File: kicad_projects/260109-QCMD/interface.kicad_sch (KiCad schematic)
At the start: 43 parts, among them J1 Conn_01x24_Socket, J2 Conn_01x24_Socket, Q1 BSS138, Q2 BSS138, Q3 BSS138, U3 LM2735YMF, U4 MIC5219-5.0YM5, U5 MIC5219-5.0YM5, U6 MIC5219-5.0YM5

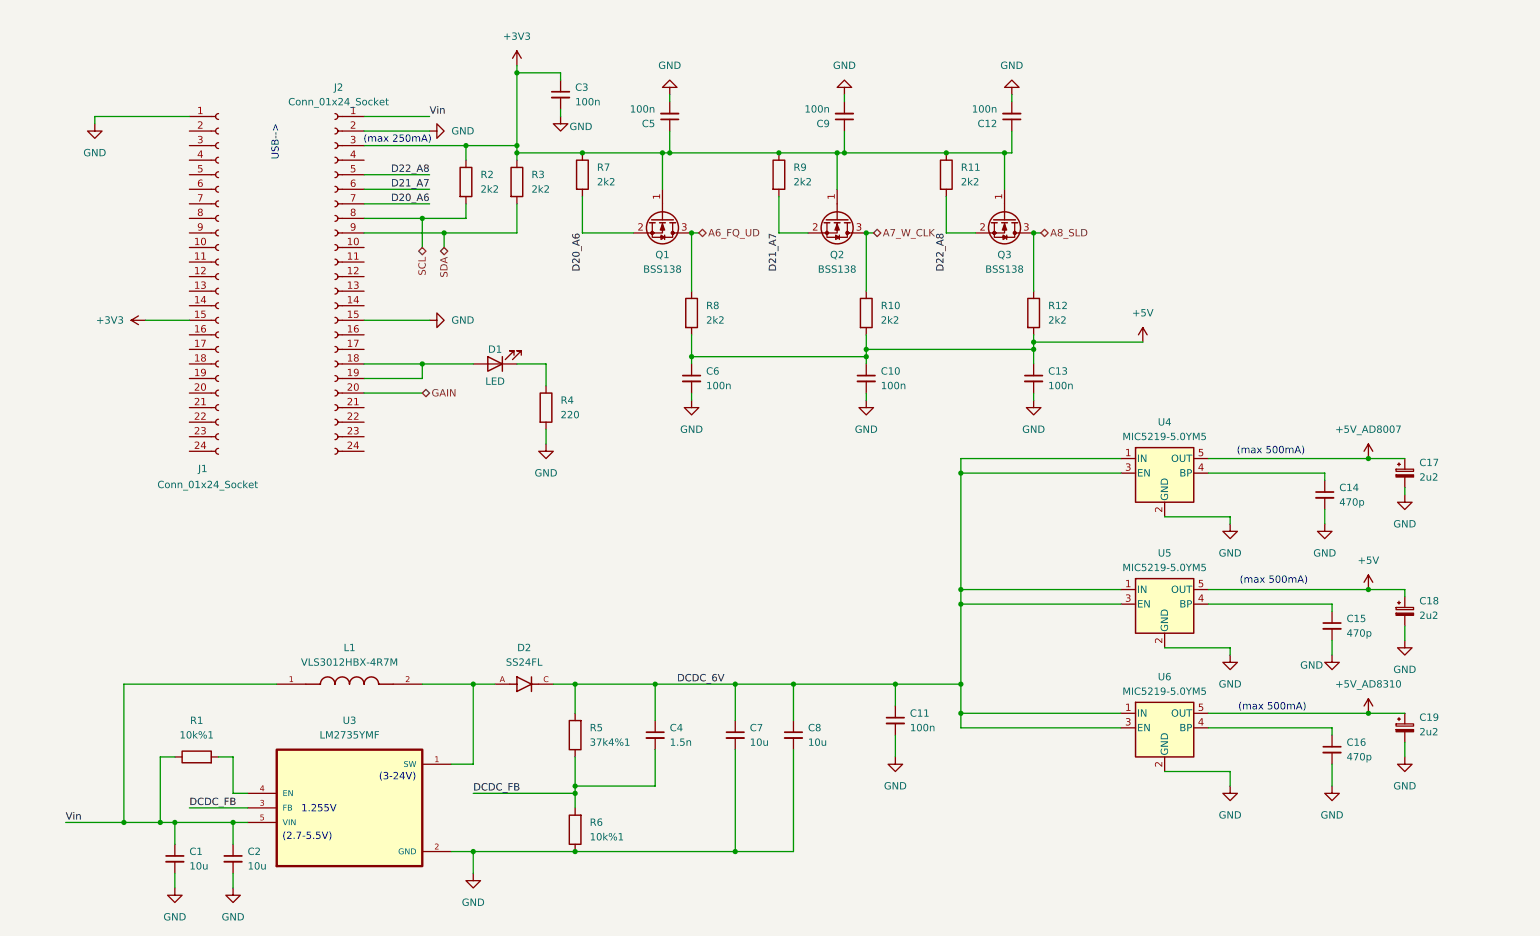
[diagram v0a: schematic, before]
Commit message: regular
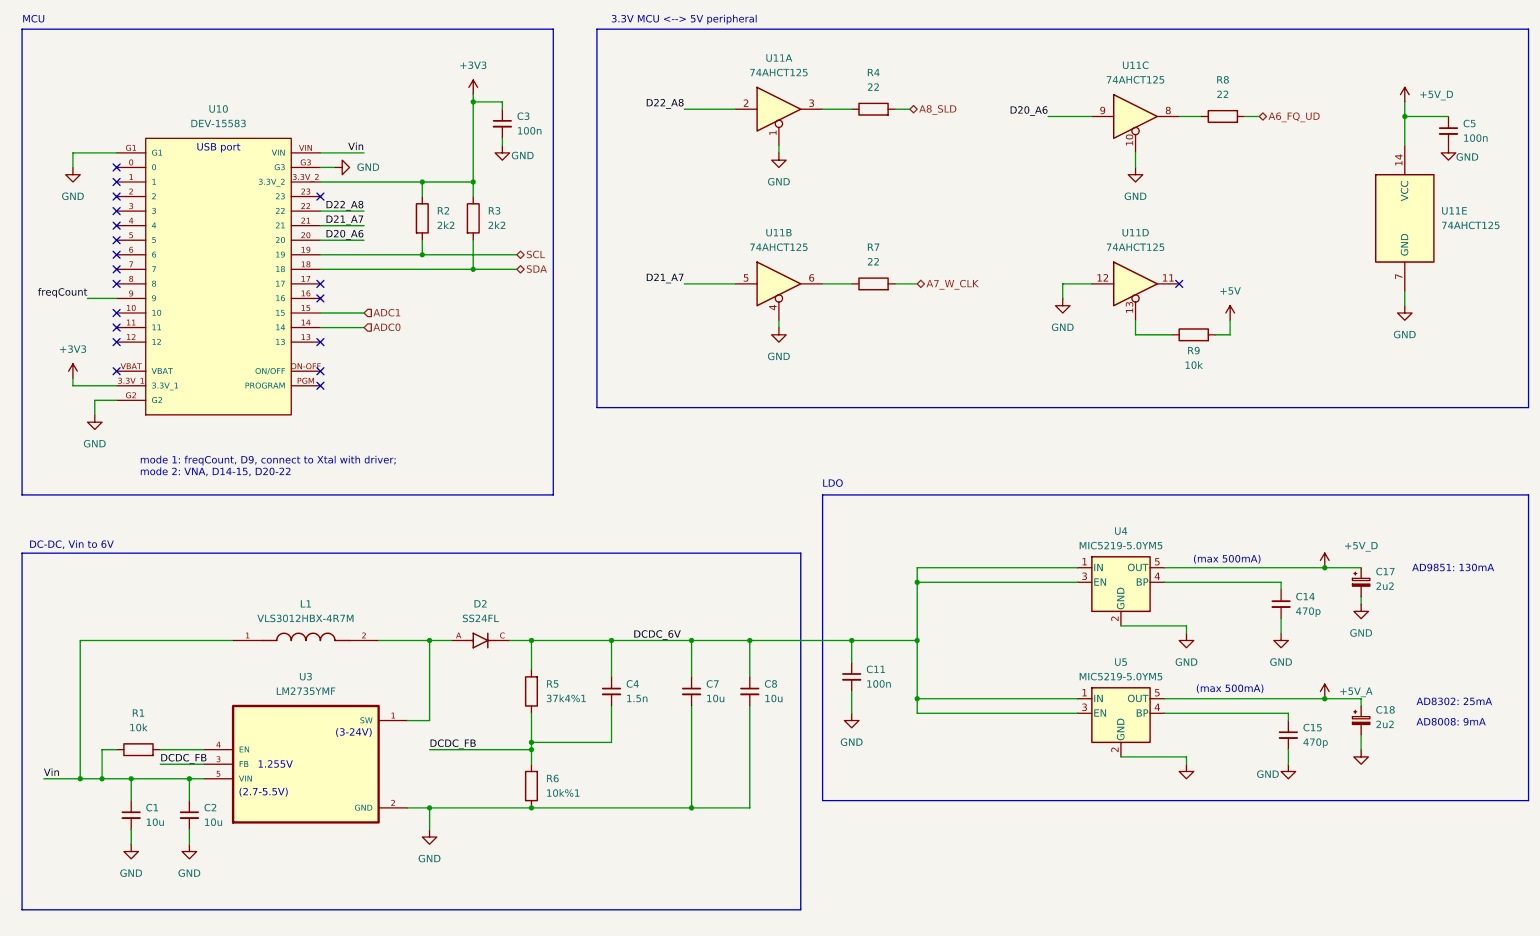
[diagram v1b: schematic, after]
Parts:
- removed C10, C12, C13, C6, C9: 100n, symbol Device:C_Small
- removed C16: 470p, symbol Device:C_Small
- removed C19: 2u2, symbol Device:C_Polarized_Small
- removed D1: LED, symbol Device:LED
- removed J1, J2: Conn_01x24_Socket, symbol Connector:Conn_01x24_Socket
- removed Q1, Q2, Q3: BSS138, Package_TO_SOT_SMD:SOT-23, symbol Transistor_FET:BSS138
- removed R10, R11, R12: 2k2, symbol Device:R
- removed U6: MIC5219-5.0YM5, Package_TO_SOT_SMD:SOT-23-5, symbol Regulator_Linear:MIC5219-5.0YM5
- added U10: DEV-15583, QCMD_footprints:DEV-15583-teensy-4, symbol DEV-15583-teensy-4:DEV-15583
- added U11: 74AHCT125, symbol 74xx:74AHCT125
- R1: value 10k%1 -> 10k
- R4: value 220 -> 22
- R7, R8: value 2k2 -> 22
- R9: value 2k2 -> 10k
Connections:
- net +3V3: now also U10.3.3V_1, U10.3.3V_2; no longer C5.1, R7.1, R9.1
- net +5V: now also R9.2; no longer C18.1, R8.2, U5.5 (OUT)
- net A6_FQ_UD: now also R8.2; no longer R8.1
- net A7_W_CLK: now also R7.2
- net A8_SLD: now also R4.2
- net D20_A6: now also U10.20, U11.9; no longer R7.2
- net D21_A7: now also U10.21, U11.5; no longer R9.2
- net D22_A8: now also U10.22, U11.2
- net GND: now also U10.G1, U10.G2, U10.G3, U11.1, U11.10, U11.12, U11.4, U11.7 (GND); no longer R4.2
- net SCL: now also U10.19
- net SDA: now also U10.18
- net Vin: now also U10.VIN
- net at R4.1: now also U11.3
- net +5V_AD8007 renamed +5V_D
- net +5V_D: now also C5.1, U11.14 (VCC)
- new net: R9.1, U11.13
- new net: R7.1, U11.6
- new net: R8.1, U11.8
- new net +5V_A: C18.1, U5.5 (OUT)
- new net ADC0: U10.14
- new net ADC1: U10.15
- new net freqCount: U10.9
- no-connect marks 0 -> 20
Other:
- note added: "3.3V MCU <--> 5V peripheral"
- note added: "AD8008: 9mA"
- note added: "AD8302: 25mA"
- note added: "AD9851: 130mA"
- note added: "DC-DC, Vin to 6V"
- note added: "LDO"
- note added: "MCU"
- note added: "USB port"
- note added: "mode 1: freqCount, D9, connect to Xtal with driver; mode 2: VNA, D14-15, D20-22"
- note removed: "(max 250mA)"
- note removed: "USB-->"
- moved on the sheet: C1, C11, C14, C15, C17, C18, C2, C3, C4, C7, C8, D2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
